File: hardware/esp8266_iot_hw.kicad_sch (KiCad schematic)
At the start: 2 parts, among them SW1 RESET, U1 NodeMCU 1.0 (ESP-12E)

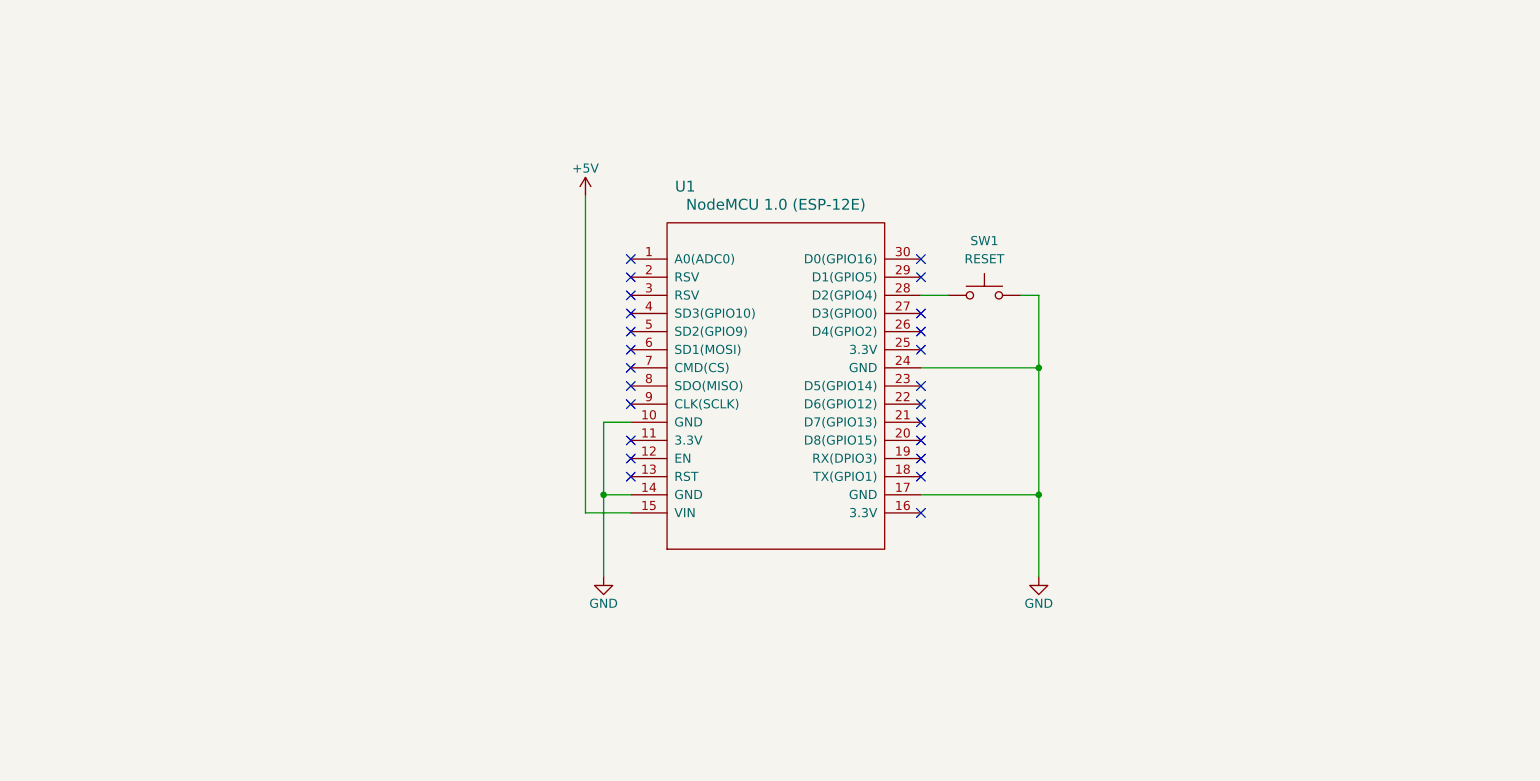
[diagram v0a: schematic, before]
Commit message: update schematics
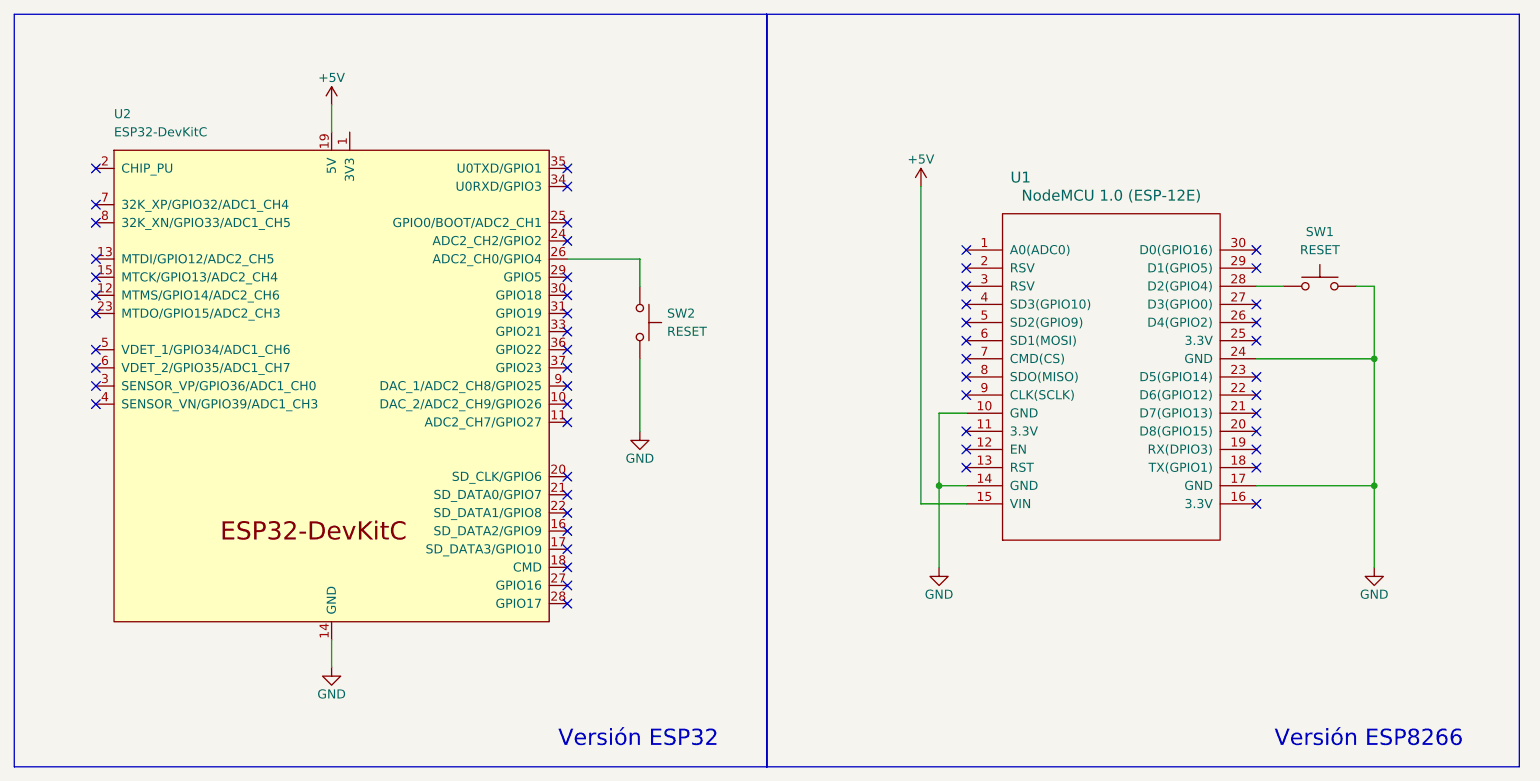
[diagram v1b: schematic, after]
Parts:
- added SW2: RESET, symbol Switch:SW_Push
- added U2: ESP32-DevKitC, PCM_Espressif:ESP32-DevKitC, symbol PCM_Espressif:ESP32-DevKitC
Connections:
- net +5V: now also U2.19 (5V)
- net GND: now also SW2.2, U2.14 (GND), U2.32 (GND), U2.38 (GND)
- new net: SW2.1, U2.26 (ADC2_CH0/GPIO4)
- no-connect marks 24 -> 56
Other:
- note added: "Versión ESP32"
- note added: "Versión ESP8266"
- title: DISPOSITIVO IOT GENERICO ESP8266 -> DISPOSITIVO IOT GENERICO ESP8266 & ESP32
- moved on the sheet: SW1, U1
